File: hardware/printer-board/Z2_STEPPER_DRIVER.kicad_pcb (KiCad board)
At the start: 2 copper layers, 7 parts, among them J11 MS_SELECT, J12 TO_MOTOR, U7 A4988_MODULE

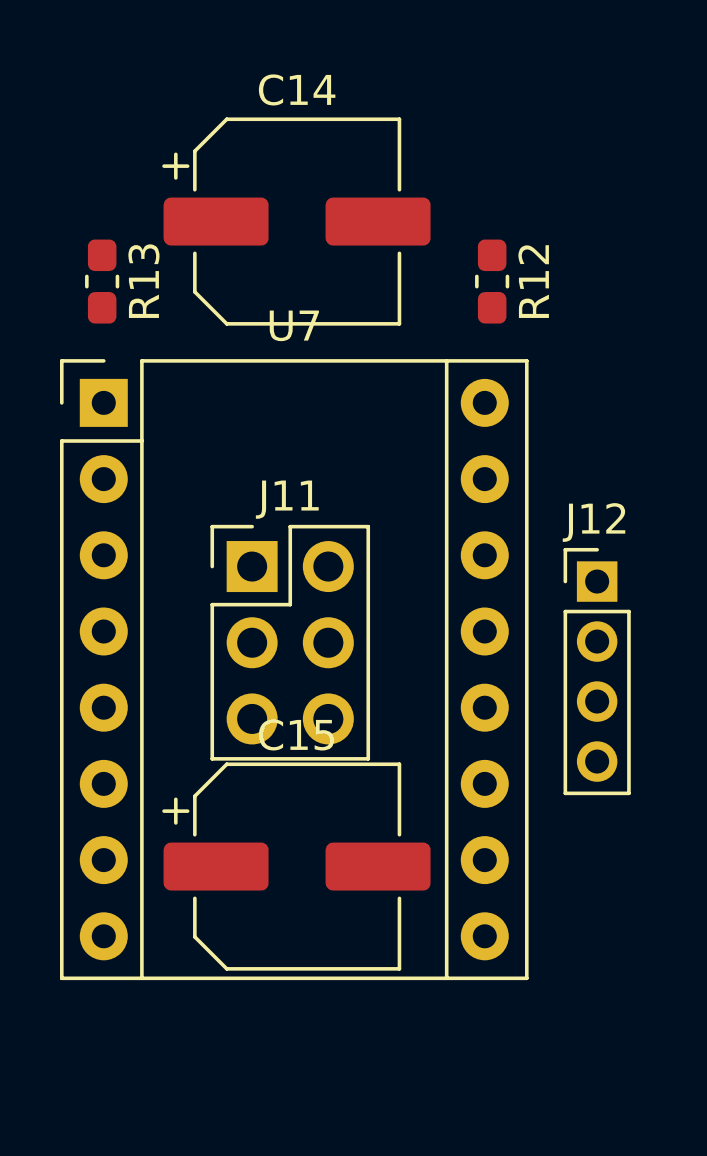
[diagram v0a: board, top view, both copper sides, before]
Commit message: update heater layouts,
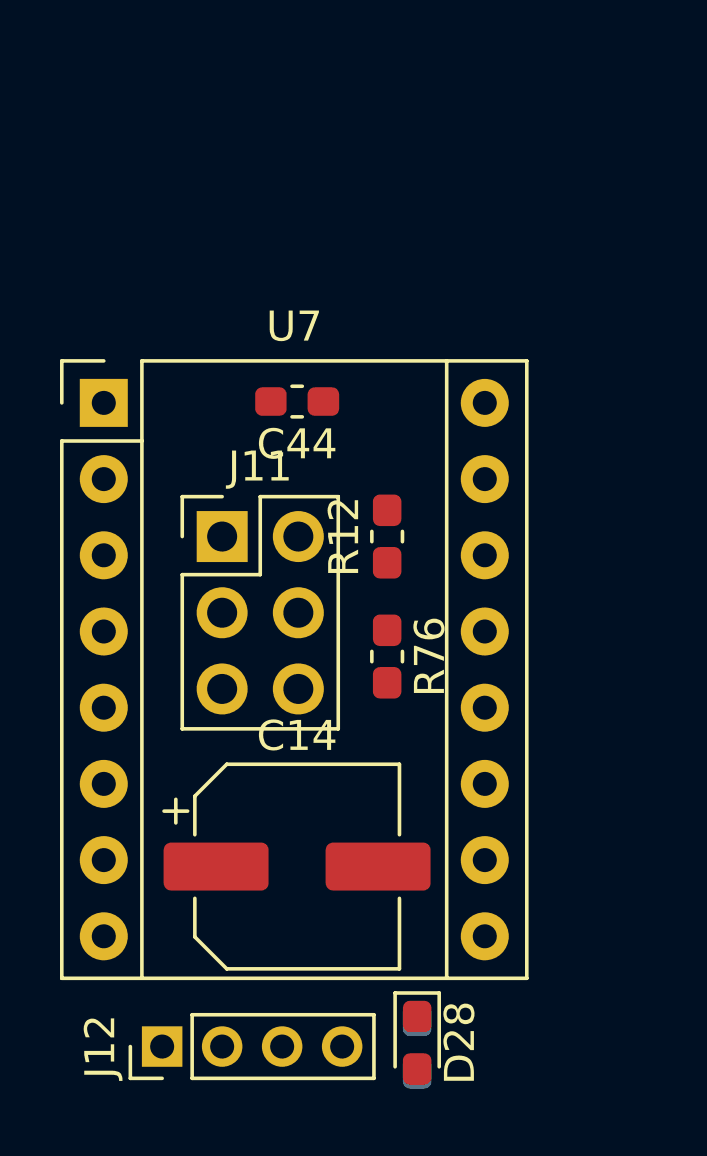
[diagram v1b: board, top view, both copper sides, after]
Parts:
- removed C15: CP100uf,25V, Capacitor_SMD:CP_Elec_6.3x7.7
- removed R13: R103,0603, Resistor_SMD:R_0603_1608Metric_Pad1.05x0.95mm_HandSolder
- added C44: C104,0603, Capacitor_SMD:C_0603_1608Metric_Pad1.05x0.95mm_HandSolder, F.Cu at (73.0, 56.5)
- added D28: LED_BLUE,0603, LED_SMD:LED_0603_1608Metric_Pad1.05x0.95mm_HandSolder, F.Cu at (77.0, 77.9)
- added R76: R102,0603, Resistor_SMD:R_0603_1608Metric_Pad1.05x0.95mm_HandSolder, F.Cu at (76.0, 65.0)
- added R77: R103,0603, Resistor_SMD:R_0603_1608Metric_Pad1.05x0.95mm_HandSolder, B.Cu at (77.0, 78.0)
- J12: value TO_MOTOR -> Z2
- moved C14 21.5 mm to (73.0, 72.0)
- moved J12 21.2 mm to (68.5, 78.0), turned to 90 degrees
- moved R12 9.19 mm to (76.0, 61.0), turned to 90 degrees
- moved J11 1.41 mm to (70.5, 61.0)
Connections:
- net +5V renamed +3V3_STM32
- net /DIR renamed /Z2_DIR
- net /STEP renamed /Z2_STEP
- U7 pad 1: /~EN~ -> /~Z2_EN~
